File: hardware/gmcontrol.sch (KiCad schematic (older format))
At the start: 0 parts

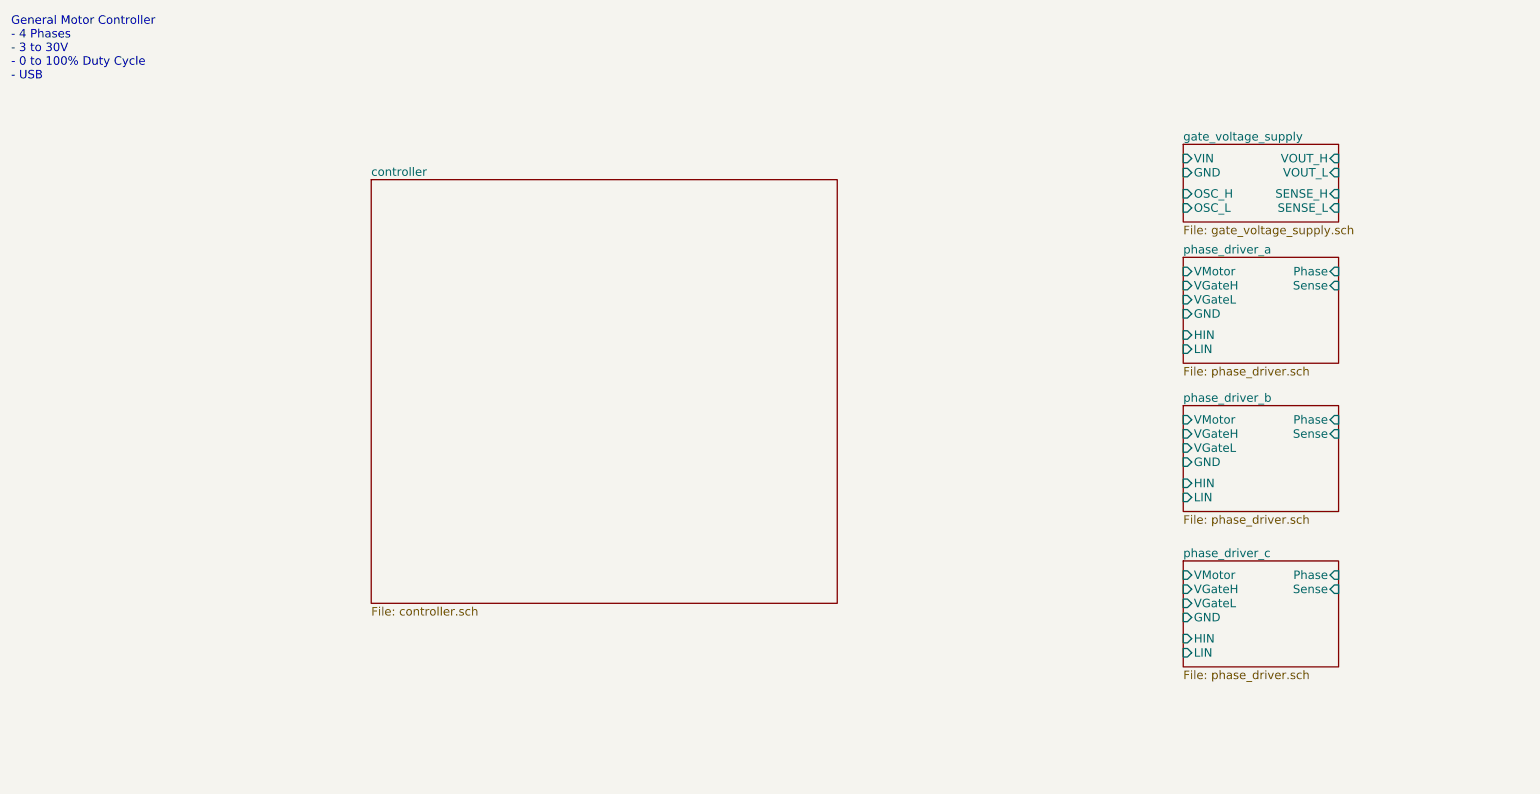
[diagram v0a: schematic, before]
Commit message: power, mcu
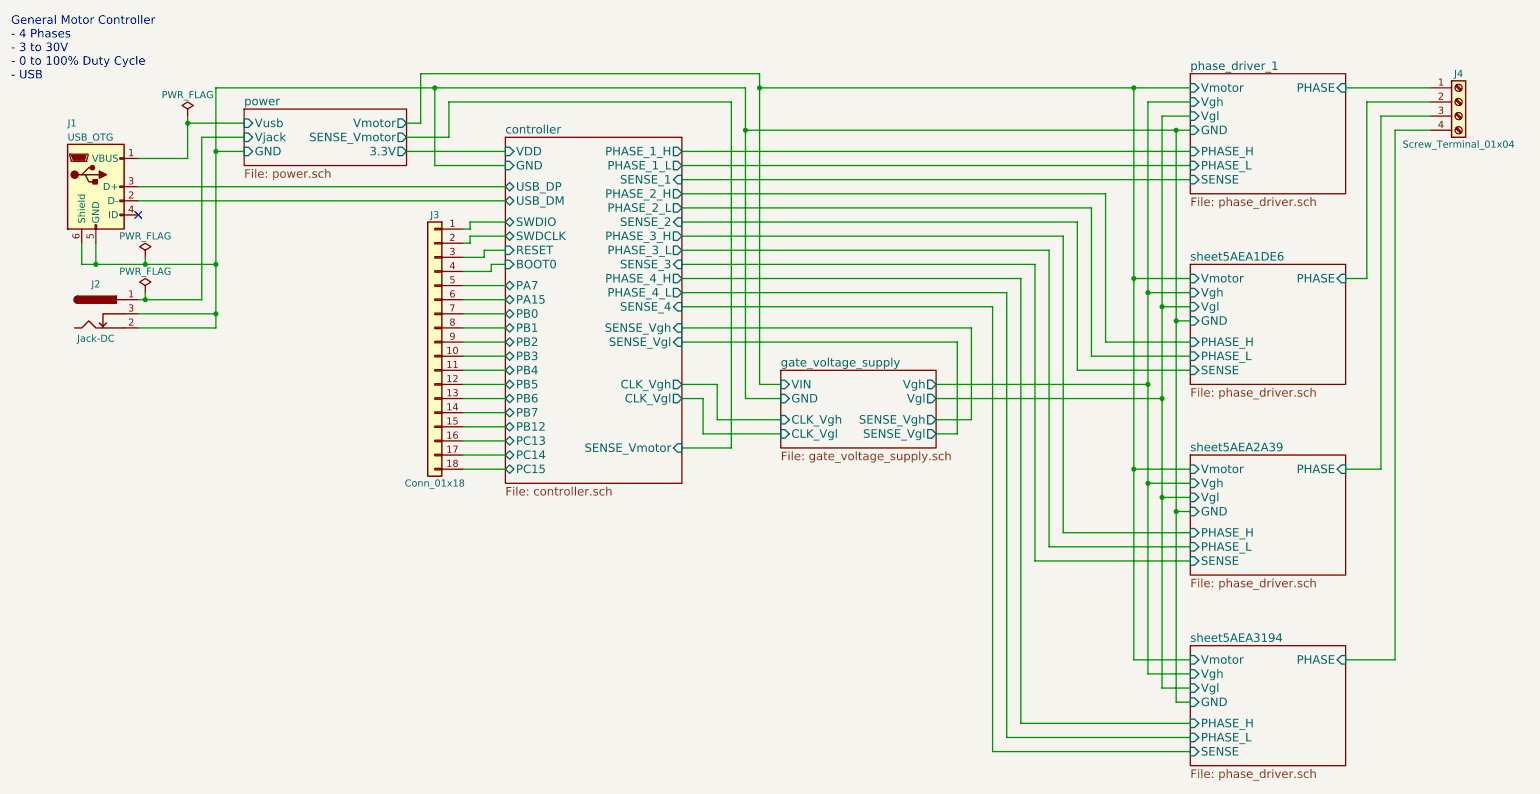
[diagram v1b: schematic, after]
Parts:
- added J1: USB_OTG, Connectors:USB_Micro-B, symbol USB_OTG
- added J2: Jack-DC, Connectors:BARREL_JACK, symbol Jack-DC
- added J3: Conn_01x18, Pin_Headers:Pin_Header_Straight_1x18_Pitch2.54mm, symbol Conn_01x18
- added J4: Screw_Terminal_01x04, Connectors_Terminal_Blocks:TerminalBlock_bornier-4_P5.08mm, symbol Screw_Terminal_01x04
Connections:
- new net controller/BOOT0: J3.4 (Pin_4)
- new net controller/GND: J1.5 (GND), J1.6 (Shield), J2.2, J2.3
- new net controller/PA15: J3.6 (Pin_6)
- new net controller/PA7: J3.5 (Pin_5)
- new net controller/PB0: J3.7 (Pin_7)
- new net controller/PB1: J3.8 (Pin_8)
- new net controller/PB12: J3.15 (Pin_15)
- new net controller/PB2: J3.9 (Pin_9)
- new net controller/PB3: J3.10 (Pin_10)
- new net controller/PB4: J3.11 (Pin_11)
- new net controller/PB5: J3.12 (Pin_12)
- new net controller/PB6: J3.13 (Pin_13)
- new net controller/PB7: J3.14 (Pin_14)
- new net controller/PC13: J3.16 (Pin_16)
- new net controller/PC14: J3.17 (Pin_17)
- new net controller/PC15: J3.18 (Pin_18)
- new net controller/RESET: J3.3 (Pin_3)
- new net controller/SWDCLK: J3.2 (Pin_2)
- new net controller/SWDIO: J3.1 (Pin_1)
- new net controller/USB_DM: J1.2 (D-)
- new net controller/USB_DP: J1.3 (D+)
- new net phase_driver_1/PHASE: J4.1 (Pin_1)
- new net power/Vjack: J2.1
- new net power/Vusb: J1.1 (VBUS)
- new net sheet5AEA1DE6/PHASE: J4.2 (Pin_2)
- new net sheet5AEA2A39/PHASE: J4.3 (Pin_3)
- new net sheet5AEA3194/PHASE: J4.4 (Pin_4)
- no-connect marks 0 -> 1

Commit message: phase routet
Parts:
- J1: footprint Connectors:USB_Micro-B -> gmcontrol:USB_Micro-B
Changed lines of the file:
@@
 F 0 "J1" H 950 2200 50  0000 L CNN
 F 1 "USB_OTG" H 950 2100 50  0000 L CNN
-F 2 "Connectors:USB_Micro-B" H 1300 1700 50  0001 C CNN
+F 2 "gmcontrol:USB_Micro-B" H 1300 1700 50  0001 C CNN
 F 3 "" H 1300 1700 50  0001 C CNN
 	1    1150 1750

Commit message: change to kicad 5
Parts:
- J1: symbol USB_OTG -> Connector:USB_B_Micro
- J2: footprint Connectors:BARREL_JACK -> Connector_BarrelJack:BarrelJack_Horizontal; symbol Jack-DC -> Connector:Jack-DC
- J3: footprint Pin_Headers:Pin_Header_Straight_1x18_Pitch2.54mm -> Connector_PinHeader_2.54mm:PinHeader_1x18_P2.54mm_Vertical; symbol Conn_01x18 -> Connector:Conn_01x18_Male
- J4: footprint Connectors_Terminal_Blocks:TerminalBlock_bornier-4_P5.08mm -> TerminalBlock:TerminalBlock_bornier-4_P5.08mm; symbol Screw_Terminal_01x04 -> Connector:Screw_Terminal_01x04
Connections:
- wire segments 133 -> 152
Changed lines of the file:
@@
-EESchema Schematic File Version 2
-LIBS:74xgxx
-LIBS:74xx
-LIBS:ac-dc
-LIBS:actel
-LIBS:adc-dac
-LIBS:allegro
-LIBS:Altera
-LIBS:analog_devices
-LIBS:analog_switches
-LIBS:atmel
-LIBS:audio
-LIBS:battery_management
-LIBS:bbd
-LIBS:bosch
-LIBS:brooktre
-LIBS:cmos4000
-LIBS:cmos_ieee
-LIBS:conn
-LIBS:contrib
-LIBS:cypress
-LIBS:dc-dc
-LIBS:device
-LIBS:digital-audio
-LIBS:diode
-LIBS:display
-LIBS:dsp
-LIBS:elec-unifil
-LIBS:ESD_Protection
-LIBS:ftdi
-LIBS:gennum
-LIBS:graphic_symbols
-LIBS:hc11
-LIBS:infineon
-LIBS:intel
-LIBS:interface
-LIBS:intersil
-LIBS:ir
-LIBS:Lattice
-LIBS:leds
-LIBS:LEM
-LIBS:linear
-LIBS:logic_programmable
-LIBS:maxim
-LIBS:mechanical
-LIBS:memory
-LIBS:microchip
-LIBS:microchip_dspic33dsc
-LIBS:microchip_pic10mcu
-LIBS:microchip_pic12mcu
-LIBS:microchip_pic16mcu
-LIBS:microchip_pic18mcu
-LIBS:microchip_pic24mcu
-LIBS:microchip_pic32mcu
-LIBS:microcontrollers
-LIBS:modules
-LIBS:motor_drivers
-LIBS:motorola
-LIBS:motors
-LIBS:msp430
-LIBS:nordicsemi
-LIBS:nxp
-LIBS:nxp_armmcu
-LIBS:onsemi
-LIBS:opto
-LIBS:Oscillators
-LIBS:philips
-LIBS:power
-LIBS:powerint
-LIBS:Power_Management
-LIBS:pspice
-LIBS:references
-LIBS:regul
-LIBS:relays
-LIBS:rfcom
-LIBS:RFSolutions
-LIBS:sensors
-LIBS:silabs
-LIBS:siliconi
-LIBS:stm8
-LIBS:stm32
-LIBS:supertex
-LIBS:switches
-LIBS:texas
-LIBS:transf
-LIBS:transistors
-LIBS:triac_thyristor
-LIBS:ttl_ieee
-LIBS:valves
-LIBS:video
-LIBS:wiznet
-LIBS:Worldsemi
-LIBS:Xicor
-LIBS:xilinx
-LIBS:zetex
-LIBS:Zilog
-LIBS:gmcontrol
+EESchema Schematic File Version 4
 LIBS:gmcontrol-cache
-EELAYER 25 0
+EELAYER 26 0
 EELAYER END
 $Descr A4 11693 8268
@@
 General Motor Controller\n- 4 Phases\n- 3 to 30V\n- 0 to 100% Duty Cycle\n- USB
 $Comp
-L USB_OTG J1
+L Connector:USB_B_Micro J1
 U 1 1 5AE89038
 P 1150 1750
@@
 $EndComp
 $Comp
-L Jack-DC J2
+L Connector:Jack-DC J2
 U 1 1 5AE89125
 P 1150 2650
 F 0 "J2" H 1150 2860 50  0000 C CNN
 F 1 "Jack-DC" H 1150 2475 50  0000 C CNN
-F 2 "Connectors:BARREL_JACK" H 1200 2610 50  0001 C CNN
+F 2 "Connector_BarrelJack:BarrelJack_Horizontal" H 1200 2610 50  0001 C CNN
 F 3 "" H 1200 2610 50  0001 C CNN
 	1    1150 2650
@@
 $EndSheet
 $Comp
-L Screw_Terminal_01x04 J4
+L Connector:Screw_Terminal_01x04 J4
 U 1 1 5AEE0660
 P 10800 1150
 F 0 "J4" H 10800 1350 50  0000 C CNN
 F 1 "Screw_Terminal_01x04" H 10800 850 50  0000 C CNN
-F 2 "Connectors_Terminal_Blocks:TerminalBlock_bornier-4_P5.08mm" H 10800 1150 50  0001 C CNN
+F 2 "TerminalBlock:TerminalBlock_bornier-4_P5.08mm" H 10800 1150 50  0001 C CNN
 F 3 "" H 10800 1150 50  0001 C CNN
 	1    10800 1150
@@
 NoConn ~ 1450 1950
 $Comp
-L Conn_01x18 J3
+L Connector:Conn_01x18_Male J3
 U 1 1 5AEF14DA
 P 3550 2850
 F 0 "J3" H 3550 3750 50  0000 C CNN
 F 1 "Conn_01x18" H 3550 1850 50  0000 C CNN
-F 2 "Pin_Headers:Pin_Header_Straight_1x18_Pitch2.54mm" H 3550 2850 50  0001 C CNN
+F 2 "Connector_PinHeader_2.54mm:PinHeader_1x18_P2.54mm_Vertical" H 3550 2850 50  0001 C CNN
 F 3 "" H 3550 2850 50  0001 C CNN
 	1    3550 2850
-	-1   0    0    -1
+	1    0    0    -1
 $EndComp
 Wire Wire Line
-	5750 1350 8900 1350
-Wire Wire Line
-	8800 1350 8800 5400
+	5750 1350 8800 1350
+Wire Wire Line
+	8800 1350 8800 2700
 Wire Wire Line
 	8800 2700 8900 2700
@@
 Connection ~ 8800 4050
 Wire Wire Line
-	8700 1250 8700 5300
+	8700 1250 8700 2600
 Wire Wire Line
 	8700 3950 8900 3950
@@
 	8900 1150 8600 1150
 Wire Wire Line
-	8600 1150 8600 5200
+	8600 1150 8600 2500
 Wire Wire Line
 	8600 2500 8900 2500
@@
 	8500 5100 8900 5100
 Wire Wire Line
-	8500 1050 8500 5100
+	8500 1050 8500 2400
 Wire Wire Line
 	8500 3750 8900 3750
@@
 	3450 950  5850 950
 Wire Wire Line
-	5850 1050 8900 1050
+	5850 1050 8500 1050
 Connection ~ 8500 2400
 Wire Wire Line
@@
 	2200 1300 1800 1300
 Wire Wire Line
-	1800 1250 1800 1550
-Wire Wire Line
 	1800 1550 1450 1550
 Wire Wire Line
 	1150 2150 1150 2300
 Wire Wire Line
-	2000 2300 1050 2300
-Wire Wire Line
-	2000 1050 2000 2750
+	2000 1050 2000 1500
 Wire Wire Line
 	2000 1500 2200 1500
@@
 Connection ~ 2000 2650
 Wire Wire Line
-	1450 2550 1900 2550
+	1450 2550 1500 2550
 Wire Wire Line
 	1900 2550 1900 1400
@@
 	5650 1150 5650 3600
 Wire Wire Line
-	5850 950  5850 3150
+	5850 950  5850 1050
 Wire Wire Line
 	5850 3150 6000 3150
 Wire Wire Line
-	2000 1050 5750 1050
-Wire Wire Line
-	5750 1050 5750 3250
+	2000 1050 3550 1050
+Wire Wire Line
+	5750 1050 5750 1350
 Wire Wire Line
 	5750 3250 6000 3250
@@
 	3750 2750 4050 2750
 Wire Wire Line
-	4050 2650 3750 2650
-Wire Wire Line
 	3750 2550 4050 2550
 Wire Wire Line
@@
 	3800 2000 4050 2000
 $Comp
-L PWR_FLAG #FLG01
-U 1 1 5AEFAA31
-P 1800 1250
-F 0 "#FLG01" H 1800 1325 50  0001 C CNN
-F 1 "PWR_FLAG" H 1800 1400 50  0000 C CNN
-F 2 "" H 1800 1250 50  0001 C CNN
-F 3 "" H 1800 1250 50  0001 C CNN
-	1    1800 1250
-	1    0    0    -1
-$EndComp
-Connection ~ 1800 1300
-$Comp
-L PWR_FLAG #FLG02
+L power:PWR_FLAG #FLG02
 U 1 1 5AEFBF25
 P 1500 2500
@@
 	1    0    0    -1
 $EndComp
-$Comp
-L PWR_FLAG #FLG03
-U 1 1 5AEFD272
-P 1500 2250
-F 0 "#FLG03" H 1500 2325 50  0001 C CNN
-F 1 "PWR_FLAG" H 1500 2400 50  0000 C CNN
-F 2 "" H 1500 2250 50  0001 C CNN
-F 3 "" H 1500 2250 50  0001 C CNN
-	1    1500 2250
-	1    0    0    -1
-$EndComp
-Wire Wire Line
-	1500 2250 1500 2300
-Connection ~ 1500 2300
 Wire Wire Line
 	1500 2500 1500 2550
 Connection ~ 1500 2550
+Wire Wire Line
+	8800 2700 8800 4050
+Wire Wire Line
+	8800 4050 8800 5400
+Wire Wire Line
+	8700 3950 8700 5300
+Wire Wire Line
+	8700 2600 8700 3250
+Wire Wire Line
+	8600 2500 8600 3150
+Wire Wire Line
+	8600 3850 8600 5200
+Wire Wire Line
+	8500 3750 8500 5100
+Wire Wire Line
+	8500 2400 8500 3750
+Wire Wire Line
+	8700 3250 8700 3950
+Wire Wire Line
+	8600 3150 8600 3850
+Wire Wire Line
+	1150 2300 1050 2300
+Wire Wire Line
+	2000 2300 2000 2650
+Wire Wire Line
+	2000 2650 2000 2750
+Wire Wire Line
+	8500 1050 8900 1050
+Wire Wire Line
+	5750 1350 5750 3250
+Wire Wire Line
+	8800 1350 8900 1350
+Wire Wire Line
+	5850 1050 5850 3150
+Wire Wire Line
+	2000 1500 2000 2300
+Wire Wire Line
+	3550 1050 5750 1050
+Wire Wire Line
+	1800 1300 1800 1550
+Wire Wire Line
+	1500 2550 1900 2550
+Wire Wire Line
+	4050 2650 3750 2650
+Wire Wire Line
+	1150 2300 2000 2300
 $EndSCHEMATC

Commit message: motor layout
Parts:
- J3: footprint Connector_PinHeader_2.54mm:PinHeader_1x18_P2.54mm_Vertical -> (none)
- J4: footprint TerminalBlock:TerminalBlock_bornier-4_P5.08mm -> (none)
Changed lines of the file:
@@
 F 0 "J4" H 10800 1350 50  0000 C CNN
 F 1 "Screw_Terminal_01x04" H 10800 850 50  0000 C CNN
-F 2 "TerminalBlock:TerminalBlock_bornier-4_P5.08mm" H 10800 1150 50  0001 C CNN
+F 2 "" H 10800 1150 50  0001 C CNN
 F 3 "" H 10800 1150 50  0001 C CNN
 	1    10800 1150
@@
 F 0 "J3" H 3550 3750 50  0000 C CNN
 F 1 "Conn_01x18" H 3550 1850 50  0000 C CNN
-F 2 "Connector_PinHeader_2.54mm:PinHeader_1x18_P2.54mm_Vertical" H 3550 2850 50  0001 C CNN
+F 2 "" H 3550 2850 50  0001 C CNN
 F 3 "" H 3550 2850 50  0001 C CNN
 	1    3550 2850
@@
 	3800 2000 4050 2000
 $Comp
-L power:PWR_FLAG #FLG02
+L power:PWR_FLAG #FLG01
 U 1 1 5AEFBF25
 P 1500 2500
-F 0 "#FLG02" H 1500 2575 50  0001 C CNN
+F 0 "#FLG01" H 1500 2575 50  0001 C CNN
 F 1 "PWR_FLAG" H 1500 2650 50  0000 C CNN
 F 2 "" H 1500 2500 50  0001 C CNN

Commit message: stm layout
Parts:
- J2: footprint Connector_BarrelJack:BarrelJack_Horizontal -> gmcontrol:BarrelJack_Horizontal_modified
- J3: footprint (none) -> Connector_PinSocket_2.54mm:PinSocket_1x18_P2.54mm_Horizontal
- J4: footprint (none) -> TerminalBlock:TerminalBlock_bornier-4_P5.08mm
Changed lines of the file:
@@
 F 0 "J2" H 1150 2860 50  0000 C CNN
 F 1 "Jack-DC" H 1150 2475 50  0000 C CNN
-F 2 "Connector_BarrelJack:BarrelJack_Horizontal" H 1200 2610 50  0001 C CNN
+F 2 "gmcontrol:BarrelJack_Horizontal_modified" H 1200 2610 50  0001 C CNN
 F 3 "" H 1200 2610 50  0001 C CNN
 	1    1150 2650
@@
 F 0 "J4" H 10800 1350 50  0000 C CNN
 F 1 "Screw_Terminal_01x04" H 10800 850 50  0000 C CNN
-F 2 "" H 10800 1150 50  0001 C CNN
+F 2 "TerminalBlock:TerminalBlock_bornier-4_P5.08mm" H 10800 1150 50  0001 C CNN
 F 3 "" H 10800 1150 50  0001 C CNN
 	1    10800 1150
@@
 F 0 "J3" H 3550 3750 50  0000 C CNN
 F 1 "Conn_01x18" H 3550 1850 50  0000 C CNN
-F 2 "" H 3550 2850 50  0001 C CNN
+F 2 "Connector_PinSocket_2.54mm:PinSocket_1x18_P2.54mm_Horizontal" H 3550 2850 50  0001 C CNN
 F 3 "" H 3550 2850 50  0001 C CNN
 	1    3550 2850

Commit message: vin
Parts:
- added MK? (x2): Mounting_Hole_PAD, MountingHole:MountingHole_2.2mm_M2_ISO7380_Pad, symbol Mechanical:Mounting_Hole_PAD
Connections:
- wire segments 152 -> 156
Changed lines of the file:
@@
 Wire Wire Line
 	1150 2300 2000 2300
+$Comp
+L Mechanical:Mounting_Hole_PAD MK?
+U 1 1 5AEFADF4
+P 1200 3200
+F 0 "MK?" V 1437 3205 50  0000 C CNN
+F 1 "Mounting_Hole_PAD" V 1346 3205 50  0000 C CNN
+F 2 "MountingHole:MountingHole_2.2mm_M2_ISO7380_Pad" H 1200 3200 50  0001 C CNN
+F 3 "" H 1200 3200 50  0001 C CNN
+	1    1200 3200
+	0    -1   -1   0
+$EndComp
+$Comp
+L Mechanical:Mounting_Hole_PAD MK?
+U 1 1 5AEFAEA3
+P 1200 3600
+F 0 "MK?" V 1437 3605 50  0000 C CNN
+F 1 "Mounting_Hole_PAD" V 1346 3605 50  0000 C CNN
+F 2 "MountingHole:MountingHole_2.2mm_M2_ISO7380_Pad" H 1200 3600 50  0001 C CNN
+F 3 "" H 1200 3600 50  0001 C CNN
+	1    1200 3600
+	0    -1   -1   0
+$EndComp
+Wire Wire Line
+	2000 2750 2000 3200
+Wire Wire Line
+	2000 3200 1300 3200
+Connection ~ 2000 2750
+Wire Wire Line
+	1300 3600 2000 3600
+Wire Wire Line
+	2000 3600 2000 3200
+Connection ~ 2000 3200
 $EndSCHEMATC

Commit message: finished pcb design
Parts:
- removed J3: Conn_01x18, Connector_PinSocket_2.54mm:PinSocket_1x18_P2.54mm_Horizontal, symbol Connector:Conn_01x18_Male
- added J10, J5, J6, J7, J8, J9: Conn_01x01, _Generic:2.54Pad, symbol Connector_Generic:Conn_01x01
- added J11, J12, J13, J14, J15, J16, J17, J18, J19, J20, J21, J22, J23, J24, J25, J26, J3: Conn_01x01, _Generic:1.27Pad, symbol Connector_Generic:Conn_01x01
- gave numbers to parts that had none: 2
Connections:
- wire segments 156 -> 160

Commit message: kicad5-stable
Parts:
- J2: symbol Connector:Jack-DC -> Connector:Barrel_Jack_Switch
- MK1, MK2: symbol Mechanical:Mounting_Hole_PAD -> Mechanical:MountingHole_Pad
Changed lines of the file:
@@
 $EndComp
 $Comp
-L Connector:Jack-DC J2
+L Connector:Barrel_Jack_Switch J2
 U 1 1 5AE89125
 P 1150 2650
@@
 	1150 2300 2000 2300
 $Comp
-L Mechanical:Mounting_Hole_PAD MK1
+L Mechanical:MountingHole_Pad MK1
 U 1 1 5AEFADF4
 P 1200 3200
@@
 $EndComp
 $Comp
-L Mechanical:Mounting_Hole_PAD MK2
+L Mechanical:MountingHole_Pad MK2
 U 1 1 5AEFAEA3
 P 1200 3600
